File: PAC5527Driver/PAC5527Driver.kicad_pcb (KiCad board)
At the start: 6 copper layers, 27.5 x 27.5 mm, 77 parts, among them J1 Conn_01x08, J2 Conn_01x04, J3 Conn_01x04, J4 Conn_01x02, U1 USBLC6-2SC6, U2 SN65HVD230, U3 MA730, U4 PAC5527, U5 HT7550-1-SOT89

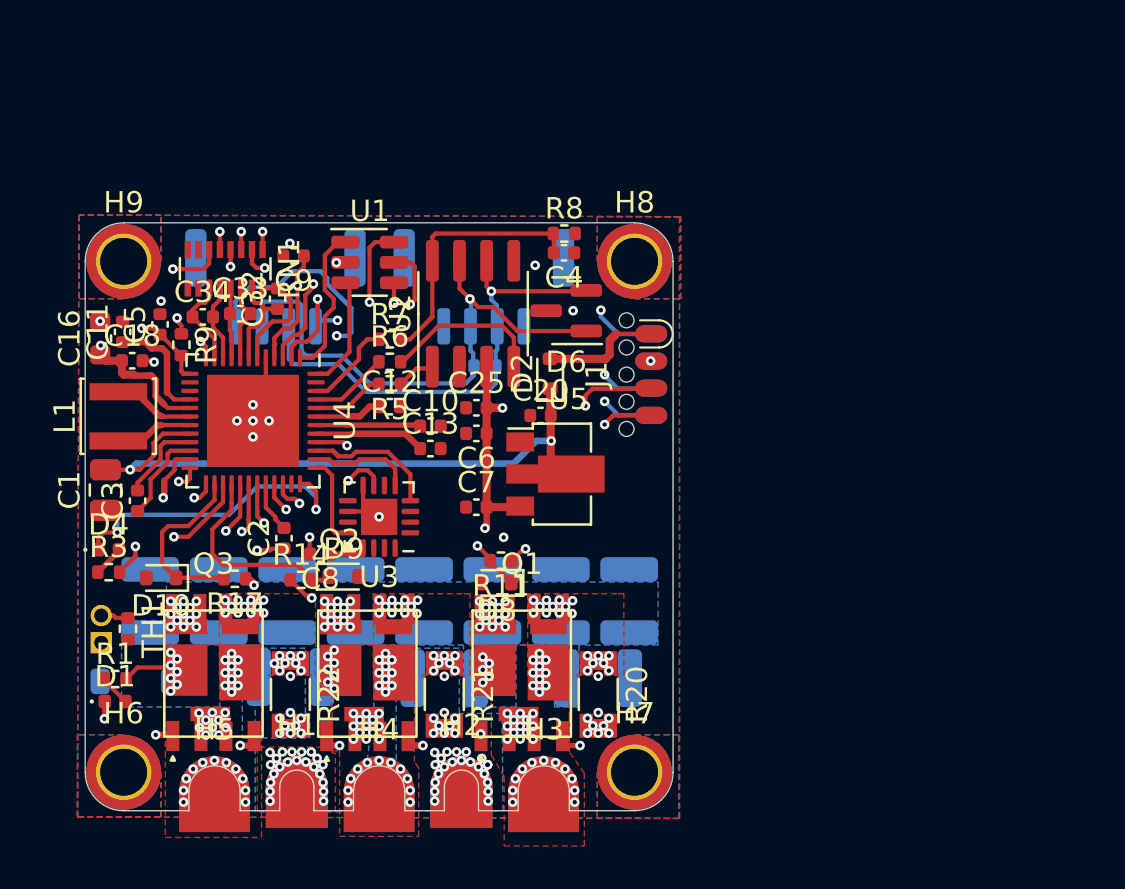
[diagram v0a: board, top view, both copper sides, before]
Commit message: redone layout
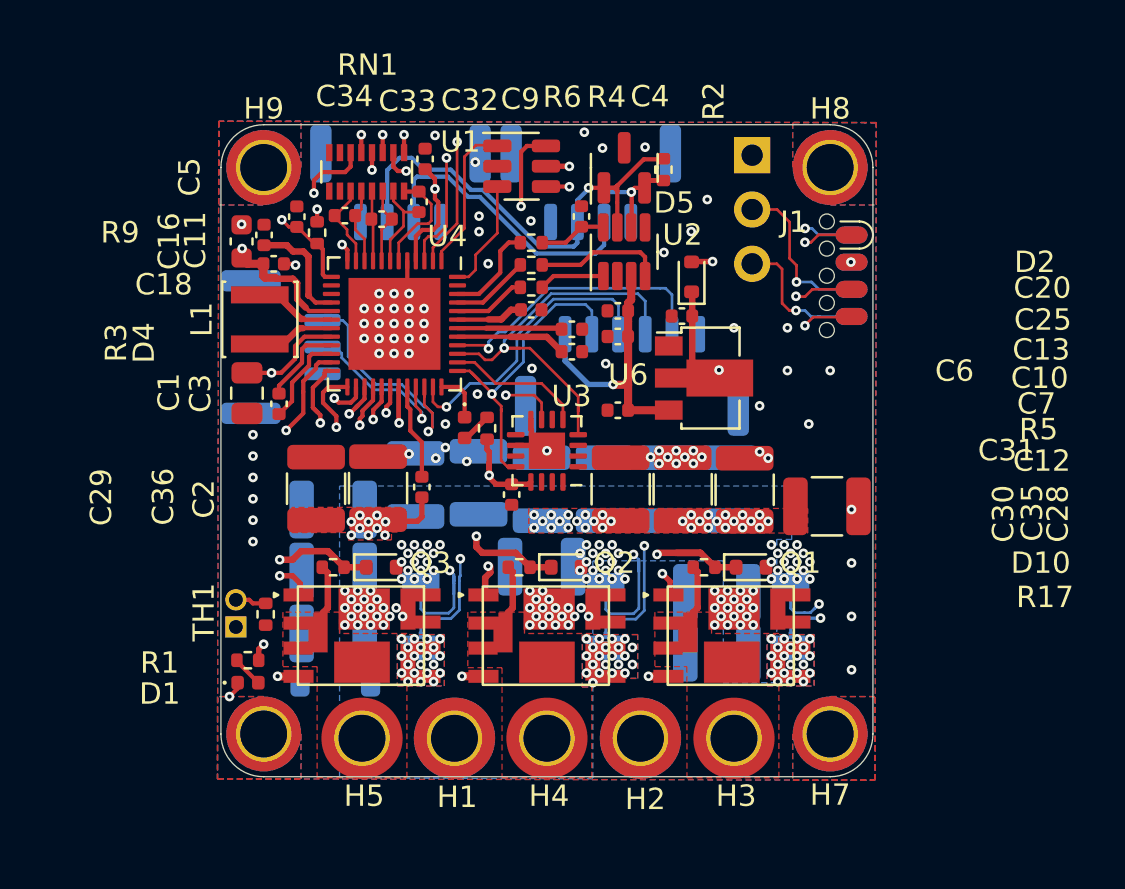
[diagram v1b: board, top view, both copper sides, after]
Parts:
- removed the C14 at (115.7, 127.4)
- removed C22, C39, C40: 10uF, Capacitor_SMD:C_1210_3225Metric
- removed D6: NUP2105L, Package_TO_SOT_SMD:SOT-23
- removed R10, R8: 10k, Resistor_SMD:R_0402_1005Metric
- removed R7: 100, Resistor_SMD:R_0402_1005Metric
- removed U5: HT7550-1-SOT89, Package_TO_SOT_SMD:SOT-89-3
- added C14: 10uF, Capacitor_SMD:C_1210_3225Metric, B.Cu at (107.1, 118.3)
- added C14: 10uF, Capacitor_SMD:C_1210_3225Metric, B.Cu at (103.2, 122.4)
- added C15: 10uF, Capacitor_SMD:C_1210_3225Metric, B.Cu at (103.2, 119.5)
- added C17: 10uF, Capacitor_SMD:C_1210_3225Metric, B.Cu at (116.0, 118.5)
- added C21: 10uF, Capacitor_SMD:C_1210_3225Metric, B.Cu at (113.0, 122.2)
- added C26: 10uF, Capacitor_SMD:C_1210_3225Metric, B.Cu at (121.2, 126.2)
- added C28: 10uF, Capacitor_SMD:C_1210_3225Metric, F.Cu at (116.7, 118.5)
- added C35: 10uF, Capacitor_SMD:C_1210_3225Metric, F.Cu at (122.5, 118.6)
- added C36: 10uF, Capacitor_SMD:C_1210_3225Metric, F.Cu at (105.3, 118.5)
- added C37: 10uF, Capacitor_SMD:C_1210_3225Metric, B.Cu at (113.0, 118.5)
- added C38: 10uF, Capacitor_SMD:C_1210_3225Metric, B.Cu at (110.0, 118.2)
- added D5: NUP2105L, Package_TO_SOT_SMD:SOT-23, F.Cu at (116.9, 103.5)
- added J5: Conn_01x06_MountingPin, Connector_JST:JST_GH_BM06B-GHS-TBT_1x06-1MP_P1.25mm_Vertical, B.Cu at (117.2, 113.2)
- added J6: Conn_01x03, Connector_PinHeader_2.54mm:PinHeader_1x03_P2.54mm_Vertical, B.Cu at (122.8, 102.9)
- added J8: Conn_01x03_MountingPin, Connector_JST:JST_GH_BM03B-GHS-TBT_1x03-1MP_P1.25mm_Vertical, B.Cu at (100.8, 111.9)
- added R2: 10k, Resistor_SMD:R_0402_1005Metric, F.Cu at (118.7, 103.6)
- added R4: 100, Resistor_SMD:R_0402_1005Metric, F.Cu at (112.5, 107.0)
- added U6: HT7533-1-SOT89, Package_TO_SOT_SMD:SOT-89-3, F.Cu at (120.9, 113.3)
- C29, C30, C31: moved to F.Cu
- H1, H2: footprint PAC5527Driver:MountingHole_SLOT_1.6_M1.5_DIN965_Pad_TopBottom -> MountingHole:MountingHole_2.2mm_M2_DIN965_Pad_TopBottom
- H3, H4, H5: footprint PAC5527Driver:MountingHole_SLOT_2.2mm_M2_DIN965_Pad_TopBottom -> MountingHole:MountingHole_2.2mm_M2_DIN965_Pad_TopOnly
- J2, J3: value Conn_01x04 -> Conn_01x04_MountingPin
- R20, R21, R22: moved to B.Cu
- R9: value 100 -> 10k
- U2: value SN65HVD230 -> TCAN330G; footprint Package_SO:SOIC-8_3.9x4.9mm_P1.27mm -> Package_TO_SOT_SMD:SOT-23-8
- moved C23 27.6 mm to (121.8, 118.5)
- moved C31 22.5 mm to (126.3, 119.3), turned to 0 degrees
- moved C27 19.7 mm to (118.8, 118.5), turned to 90 degrees
- moved R3 18.9 mm to (110.5, 115.7), turned to -90 degrees
- moved D4 17.6 mm to (109.4, 115.7), turned to -90 degrees
- moved C24 13.4 mm to (121.2, 123.4)
- moved C30 13.2 mm to (119.6, 118.5)
- moved D8 11.9 mm to (122.8, 122.2), turned to 0 degrees
- moved J1 10.4 mm to (128.2, 108.6)
- moved D9 10.4 mm to (114.2, 122.2)
- moved D10 10.3 mm to (105.5, 122.2), turned to 0 degrees
- moved R14 10.2 mm to (112.0, 122.2)
- moved H8 10.1 mm to (126.5, 103.5)
- moved Q1 9.98 mm to (121.9, 125.4), turned to -90 degrees
- moved C29 9.78 mm to (102.5, 118.5)
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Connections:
- C4 pad 1: GND -> Net-(U2-S)
- C4 pad 2: Net-(U2-Rs) -> GND
- J2 pad 1: unconnected-(J2-Pin_1-Pad1) -> GND
- J2 pad MP: (no net) -> GND
- J3 pad 1: /MB_ID_0 -> GND
- J3 pad 4: /MB_ID_1 -> unconnected-(J3-Pin_4-Pad4)
- J3 pad MP: (no net) -> GND
- U2 pad 8: Net-(U2-Rs) -> Net-(U2-S)
- U4 pad 35: unconnected-(U4D-PD5-Pad35) -> /ENC_CS1
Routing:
- net /ENC_CS1: track 0.00 -> 13.7 mm, vias 0 -> 1
- net /ENC_MISO: track 5.12 -> 18.5 mm
- net /MB_ID_0: track 22.1 -> 8.86 mm, vias 2 -> 1
- net /ENC_MOSI: track 6.65 -> 19.4 mm, vias 0 -> 1
- net Net-(U2-Rs): track 12.6 -> 0.00 mm
- net /LED_IN: track 14.9 -> 2.33 mm, vias 2 -> 0
- net /VL: track 33.2 -> 21.3 mm
- net /ENC_SCLK: track 4.23 -> 15.1 mm, vias 0 -> 1
- net /WS: track 8.51 -> 16.2 mm, vias 0 -> 2
- net /SWDCL: track 24.6 -> 31.3 mm
- net /EXT_UART_RX: track 14.9 -> 21.5 mm
- net /US: track 17.4 -> 23.7 mm
- net /PBTN: track 35.2 -> 29.1 mm
- net /VS: track 9.66 -> 15.3 mm, vias 0 -> 2
- net /EXT_UART_TX: track 19.8 -> 25.4 mm
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- added copper zone on B.Cu, net Net-(Q1-PadSL)
- added copper zone on B.Cu, net Net-(Q2-PadSL)
- added copper zone on B.Cu, net Net-(Q3-PadSL)
- added copper zone on In3.Cu, net VDC
- removed copper zone on In1.Cu, net /UOUT
- removed copper zone on In2.Cu, net /UOUT
- removed copper zone on In1.Cu, net /VOUT
- removed copper zone on In2.Cu, net /VOUT
- removed copper zone on In1.Cu, net /WOUT
- removed copper zone on In2.Cu, net /WOUT
- removed copper zone on In1.Cu, net Net-(Q1-PadSL)
- removed copper zone on In2.Cu, net Net-(Q1-PadSL)
- removed copper zone on In1.Cu, net Net-(Q2-PadSL)
- removed copper zone on In2.Cu, net Net-(Q2-PadSL)
- removed copper zone on In1.Cu, net Net-(Q3-PadSL)
- removed copper zone on In2.Cu, net Net-(Q3-PadSL)
- removed copper zone on In4.Cu, net VDC
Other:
- board size 27.5 x 27.5 mm -> 30.5 x 30.5 mm
